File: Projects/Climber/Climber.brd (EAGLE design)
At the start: 160 x 100 mm, 3 parts, among them M1 VNH5019, M2 D36V6FX, U1 NRF52840-DONGLE

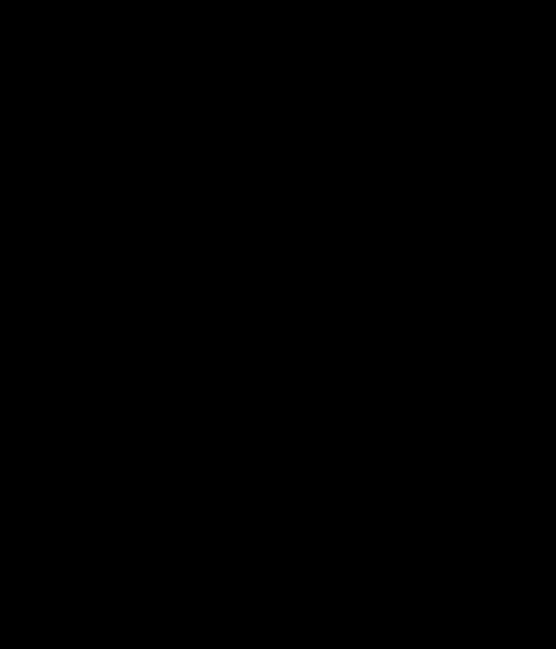
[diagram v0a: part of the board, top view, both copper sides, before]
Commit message: New devices in Climber
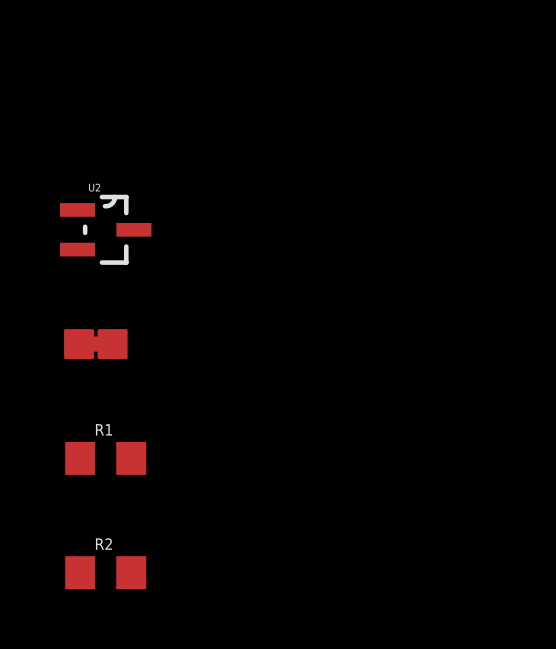
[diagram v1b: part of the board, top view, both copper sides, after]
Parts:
- added R1, R2: (no value), resistor:R0603
- added U$10: NET_CONN, NET_CONN:NET_CONN
- added U2: BSS138BKW, BSS138:SOT65P210X110-3N
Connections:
- net VOUT renamed M1_VOUT
- new net M1_CS: M1.CS
- new net M1_ENA/DIAGA: M1.ENA
- new net M1_ENB/DIAGB: M1.ENB
- new net M1_INA: M1.INA
- new net M1_INB: M1.INB
- new net M1_PWM: M1.PWM
- new net NEO_HV: R2.1, U2.3
- new net NEO_LV: R1.1, U2.2
- new net VDD_5V: R2.2
- net GND: now also U$10.1, U$10.2
- net VDD: now also M2.VOUT, R1.2, U1.OUT
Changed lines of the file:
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@@
 <layer number="111" name="LPC17xx" color="7" fill="1" visible="yes" active="yes"/>
 <layer number="112" name="tSilk" color="7" fill="1" visible="yes" active="yes"/>
+<layer number="113" name="FRNTTEKEN" color="7" fill="1" visible="yes" active="yes"/>
+<layer number="114" name="FRNTMAAT1" color="7" fill="1" visible="yes" active="yes"/>
+<layer number="115" name="FRNTMAAT2" color="7" fill="1" visible="yes" active="yes"/>
 <layer number="116" name="Patch_BOT" color="9" fill="4" visible="yes" active="yes"/>
+<layer number="117" name="BACKMAAT1" color="7" fill="1" visible="yes" active="yes"/>
+<layer number="118" name="BACKMAAT2" color="7" fill="1" visible="yes" active="yes"/>
+<layer number="119" name="KAP_TEKEN" color="7" fill="1" visible="yes" active="yes"/>
 <layer number="120" name="_Dimension" color="7" fill="1" visible="yes" active="yes"/>
 <layer number="121" name="_tsilk" color="6" fill="1" visible="yes" active="yes"/>
@@
 <layer number="127" name="_tValues" color="6" fill="1" visible="yes" active="yes"/>
 <layer number="128" name="_bValues" color="6" fill="1" visible="yes" active="yes"/>
+<layer number="130" name="SMDSTROOK" color="7" fill="1" visible="yes" active="yes"/>
 <layer number="131" name="tAdjust" color="7" fill="1" visible="yes" active="yes"/>
 <layer number="132" name="bAdjust" color="7" fill="1" visible="yes" active="yes"/>
@@
 <layer number="251" name="bxdocu" color="7" fill="1" visible="no" active="yes"/>
 <layer number="254" name="cooling" color="7" fill="1" visible="yes" active="yes"/>
+<layer number="255" name="Accent" color="7" fill="1" visible="yes" active="yes"/>
 </layers>
 <board>
@@
 <attribute name="VALUE" x="30.9626" y="59.69" size="1.27" layer="27" rot="R180"/>
 </element>
+<element name="U2" library="BSS138" package="SOT65P210X110-3N" value="BSS138BKW" x="-17.78" y="2.54" smashed="yes">
+<attribute name="MPN" value="BSS138BKW" x="-17.78" y="2.54" size="1.778" layer="27" display="off"/>
+<attribute name="NAME" x="-18.3642" y="3.8196" size="0.254" layer="25" ratio="10" rot="SR0"/>
+<attribute name="OC_FARNELL" value="2053836" x="-17.78" y="2.54" size="1.778" layer="27" display="off"/>
+<attribute name="OC_NEWARK" value="61T7488" x="-17.78" y="2.54" size="1.778" layer="27" display="off"/>
+<attribute name="PACKAGE" value="SOT-23-3" x="-17.78" y="2.54" size="1.778" layer="27" display="off"/>
+<attribute name="SUPPLIER" value="NXP" x="-17.78" y="2.54" size="1.778" layer="27" display="off"/>
+<attribute name="VALUE" x="-18.3642" y="1.043" size="0.254" layer="27" ratio="10" rot="SR0"/>
+</element>
+<element name="U$10" library="NET_CONN" package="NET_CONN" value="NET_CONN" x="-19.05" y="-1.27" smashed="yes"/>
+<element name="R1" library="resistor" package="R0603" value="" x="-17.78" y="-5.08" smashed="yes">
+<attribute name="NAME" x="-17.526" y="-3.937" size="0.381" layer="25" rot="R180"/>
+<attribute name="VALUE" x="-19.304" y="-6.223" size="0.381" layer="27"/>
+</element>
+<element name="R2" library="resistor" package="R0603" value="" x="-17.78" y="-8.89" smashed="yes">
+<attribute name="NAME" x="-17.526" y="-7.747" size="0.381" layer="25" rot="R180"/>
+<attribute name="VALUE" x="-19.304" y="-10.033" size="0.381" layer="27"/>
+</element>
 </elements>
 <signals>
 <signal name="VDD">
 <contactref element="M1" pad="VDD"/>
+<contactref element="M2" pad="VOUT"/>
+<contactref element="U1" pad="OUT"/>
+<contactref element="R1" pad="2"/>
+<wire x1="44.45" y1="83.82" x2="57.15" y2="86.36" width="0" layer="19" extent="1-1"/>
+<wire x1="5.0876" y1="57.15" x2="44.45" y2="83.82" width="0" layer="19" extent="1-1"/>
+<wire x1="-16.93" y1="-5.08" x2="5.0876" y2="57.15" width="0" layer="19" extent="1-1"/>
 </signal>
 <signal name="GND">
 <contactref element="M1" pad="GND@0"/>
 <contactref element="M1" pad="GND@1"/>
+<contactref element="U1" pad="G3"/>
+<contactref element="U1" pad="G1"/>
+<contactref element="U1" pad="G2"/>
+<contactref element="U$10" pad="1"/>
+<contactref element="U$10" pad="2"/>
 <contactref element="M2" pad="GND"/>
-<contactref element="U1" pad="G1"/>
-<contactref element="U1" pad="G3"/>
-<contactref element="U1" pad="G2"/>
 <wire x1="44.45" y1="86.36" x2="59.69" y2="86.36" width="0" layer="19" extent="1-1"/>
 <wire x1="44.45" y1="91.44" x2="44.45" y2="86.36" width="0" layer="19" extent="1-1"/>
-<wire x1="25.4076" y1="41.91" x2="44.45" y2="86.36" width="0" layer="19" extent="1-1"/>
-<wire x1="25.4076" y1="57.15" x2="25.4076" y2="41.91" width="0" layer="19" extent="1-1"/>
+<wire x1="25.4076" y1="57.15" x2="44.45" y2="86.36" width="0" layer="19" extent="1-1"/>
+<wire x1="25.4076" y1="41.91" x2="25.4076" y2="57.15" width="0" layer="19" extent="1-1"/>
 <wire x1="7.6276" y1="57.15" x2="25.4076" y2="57.15" width="0" layer="19" extent="1-1"/>
-</signal>
-<signal name="VOUT">
-<contactref element="M1" pad="VOUT"/>
+<wire x1="-17.55" y1="-1.27" x2="25.4076" y2="41.91" width="0" layer="19" extent="1-1"/>
+<wire x1="-18.669" y1="-1.27" x2="-17.55" y2="-1.27" width="0" layer="19" extent="1-1"/>
 </signal>
 <signal name="VIN">
@@
 <contactref element="U1" pad="VBUS"/>
 </signal>
+<signal name="NEO_LV">
+<contactref element="R1" pad="1"/>
+<contactref element="U2" pad="2"/>
+<wire x1="-18.7198" y1="1.8796" x2="-18.63" y2="-5.08" width="0" layer="19" extent="1-1"/>
+</signal>
+<signal name="NEO_HV">
+<contactref element="U2" pad="3"/>
+<contactref element="R2" pad="1"/>
+<wire x1="-16.8402" y1="2.54" x2="-18.63" y2="-8.89" width="0" layer="19" extent="1-1"/>
+</signal>
+<signal name="VDD_5V">
+<contactref element="R2" pad="2"/>
+</signal>
+<signal name="M1_INA">
+<contactref element="M1" pad="INA"/>
+</signal>
+<signal name="M1_INB">
+<contactref element="M1" pad="INB"/>
+</signal>
+<signal name="M1_ENA/DIAGA">
+<contactref element="M1" pad="ENA"/>
+</signal>
+<signal name="M1_ENB/DIAGB">
+<contactref element="M1" pad="ENB"/>
+</signal>
+<signal name="M1_PWM">
+<contactref element="M1" pad="PWM"/>
+</signal>
+<signal name="M1_VOUT">
+<contactref element="M1" pad="VOUT"/>
+</signal>
+<signal name="M1_CS">
+<contactref element="M1" pad="CS"/>
+</signal>
 </signals>
